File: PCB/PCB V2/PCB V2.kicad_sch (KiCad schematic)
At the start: 57 parts, among them J1 Screw_Terminal_01x03, J2 Screw_Terminal_01x03, J3 USB_B, J4 Conn_01x02_Pin, K1 Relay_SPDT, K2 Relay_SPDT, Q1 S8050, Q2 S8050, Q3 S8050, SW1 On/Off, SW2 SW_Push, SW3 SW_Push, U1 LM317_TO-220, U2 LM317_TO-220

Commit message: Cambiado el footprint del capacitor
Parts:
- C1, C4: footprint Capacitor_THT:CP_Radial_D10.0mm_P3.50mm -> Capacitor_THT:CP_Radial_D6.3mm_P2.50mm
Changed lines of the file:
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@@
 			)
 		)
-		(property "Footprint" "Capacitor_THT:CP_Radial_D10.0mm_P3.50mm"
+		(property "Footprint" "Capacitor_THT:CP_Radial_D6.3mm_P2.50mm"
 			(at 227.0252 110.49 0)
 			(effects
@@
 			)
 		)
-		(property "Footprint" "Capacitor_THT:CP_Radial_D10.0mm_P3.50mm"
+		(property "Footprint" "Capacitor_THT:CP_Radial_D6.3mm_P2.50mm"
 			(at 224.4852 80.01 0)
 			(effects

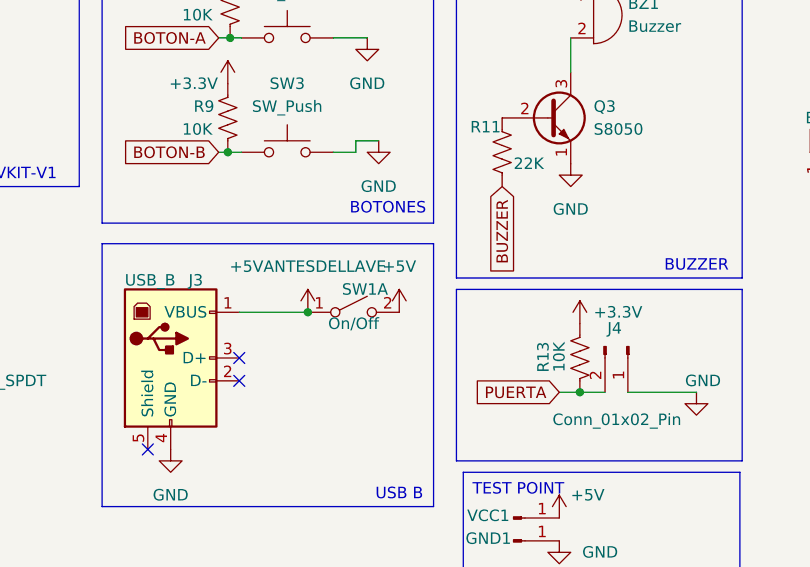
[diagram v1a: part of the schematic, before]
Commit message: .
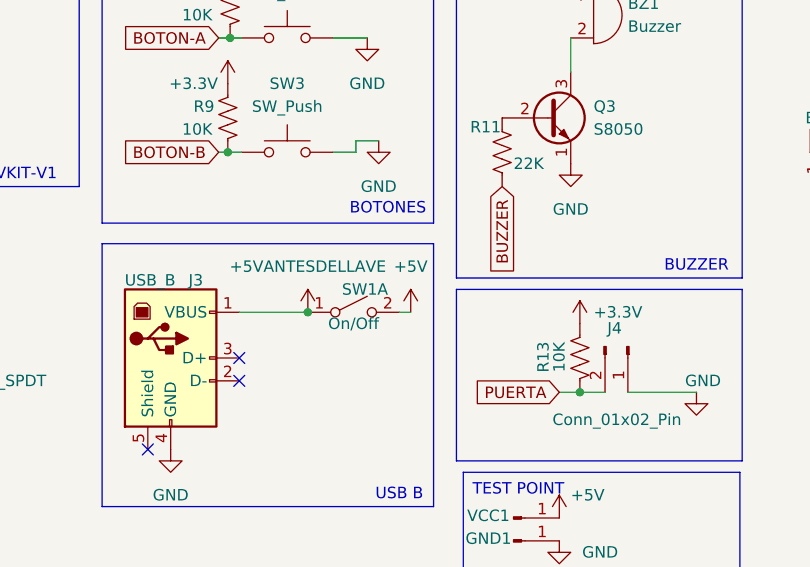
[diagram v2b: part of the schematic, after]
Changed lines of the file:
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@@
 	(wire
 		(pts
+			(xy 175.26 105.41) (xy 173.99 105.41)
+		)
+		(stroke
+			(width 0)
+			(type default)
+		)
+	)
+	(wire
+		(pts
 			(xy 256.54 95.25) (xy 247.65 95.25)
 		)
@@
 	(symbol
 		(lib_id "power:+5V")
-		(at 173.99 105.41 0)
+		(at 175.26 105.41 0)
 		(unit 1)
 		(exclude_from_sim no)
@@
 		(fields_autoplaced yes)
 		(property "Reference" "#PWR026"
-			(at 173.99 109.22 0)
+			(at 175.26 109.22 0)
 			(effects
 				(font
@@
 		)
 		(property "Value" "+5V"
-			(at 173.99 100.33 0)
+			(at 175.26 100.33 0)
 			(effects
 				(font
@@
 		)
 		(property "Footprint" ""
-			(at 173.99 105.41 0)
+			(at 175.26 105.41 0)
 			(effects
 				(font
@@
 		)
 		(property "Datasheet" ""
-			(at 173.99 105.41 0)
+			(at 175.26 105.41 0)
 			(effects
 				(font
@@
 		)
 		(property "Description" "Power symbol creates a global label with name \"+5V\""
-			(at 173.99 105.41 0)
+			(at 175.26 105.41 0)
 			(effects
 				(font

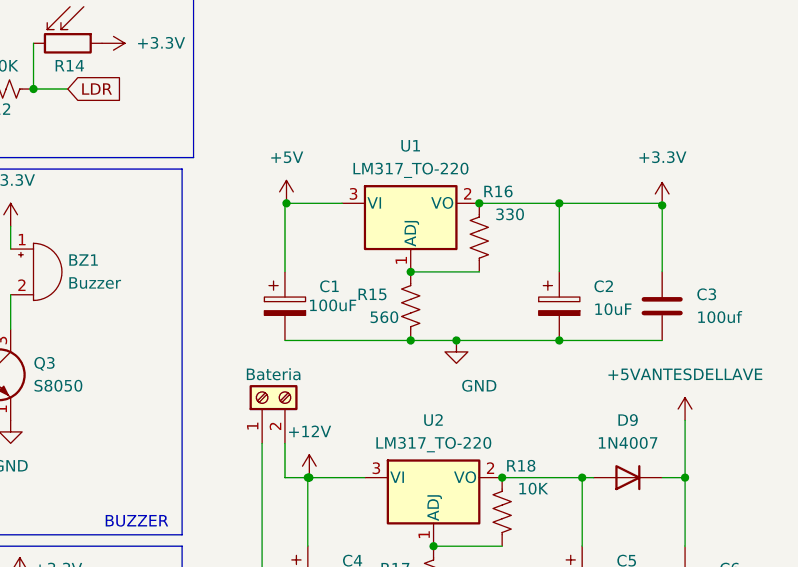
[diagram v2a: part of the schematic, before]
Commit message: .
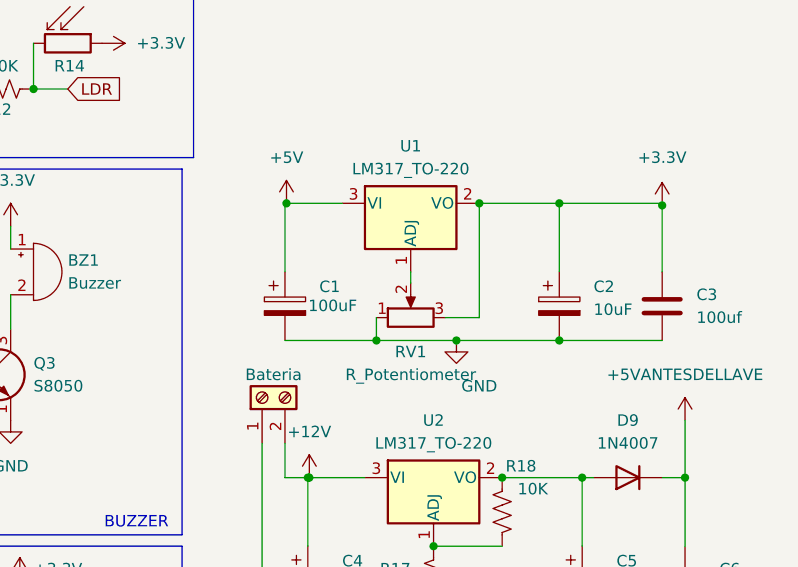
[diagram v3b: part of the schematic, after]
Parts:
- removed R15: 560, Resistor_THT:R_Axial_DIN0207_L6.3mm_D2.5mm_P10.16mm_Horizontal, symbol Device:R_US
- removed R16: 330, Resistor_THT:R_Axial_DIN0207_L6.3mm_D2.5mm_P10.16mm_Horizontal, symbol Device:R_US
- added RV1: R_Potentiometer, Potentiometer_THT:Potentiometer_Bourns_3386W_Horizontal, symbol Device:R_Potentiometer
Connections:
- net +3.3V: now also RV1.3
- net GND: now also RV1.1
- net at U1.1 (ADJ): now also RV1.2
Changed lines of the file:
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@@
 	)
 	(junction
+		(at 233.68 80.01)
+		(diameter 0)
+		(color 0 0 0 0)
+	)
+	(junction
 		(at 45.72 118.11)
 		(diameter 0)
@@
 	)
 	(junction
-		(at 245.11 64.77)
-		(diameter 0)
-		(color 0 0 0 0)
-	)
-	(junction
 		(at 97.79 119.38)
 		(diameter 0)
@@
 	)
 	(junction
-		(at 237.49 72.39)
-		(diameter 0)
-		(color 0 0 0 0)
-	)
-	(junction
 		(at 247.65 95.25)
 		(diameter 0)
@@
 	)
 	(junction
-		(at 237.49 80.01)
+		(at 245.11 64.77)
 		(diameter 0)
 		(color 0 0 0 0)
@@
 	(wire
 		(pts
+			(xy 233.68 80.01) (xy 242.57 80.01)
+		)
+		(stroke
+			(width 0)
+			(type default)
+		)
+	)
+	(wire
+		(pts
 			(xy 165.2503 28.535) (xy 157.6303 28.535)
 		)
@@
 	(wire
 		(pts
-			(xy 237.49 80.01) (xy 242.57 80.01)
+			(xy 223.52 80.01) (xy 233.68 80.01)
 		)
 		(stroke
@@
 	(wire
 		(pts
-			(xy 223.52 80.01) (xy 237.49 80.01)
-		)
-		(stroke
-			(width 0)
-			(type default)
-		)
-	)
-	(wire
-		(pts
 			(xy 166.5203 31.075) (xy 165.2503 31.075)
 		)
@@
 	(wire
 		(pts
-			(xy 237.49 72.39) (xy 245.11 72.39)
-		)
-		(stroke
-			(width 0)
-			(type default)
-		)
-	)
-	(wire
-		(pts
 			(xy 60.96 118.11) (xy 66.04 118.11)
 		)
@@
 	(wire
 		(pts
+			(xy 245.11 64.77) (xy 245.11 77.47)
+		)
+		(stroke
+			(width 0)
+			(type default)
+		)
+	)
+	(wire
+		(pts
+			(xy 237.49 73.66) (xy 237.49 72.39)
+		)
+		(stroke
+			(width 0)
+			(type default)
+		)
+	)
+	(wire
+		(pts
+			(xy 233.68 77.47) (xy 233.68 80.01)
+		)
+		(stroke
+			(width 0)
+			(type default)
+		)
+	)
+	(wire
+		(pts
+			(xy 241.3 77.47) (xy 245.11 77.47)
+		)
+		(stroke
+			(width 0)
+			(type default)
+		)
+	)
+	(wire
+		(pts
 			(xy 223.686 64.77) (xy 223.52 64.77)
 		)
@@
 	)
 	(symbol
-		(lib_id "Device:R_US")
-		(at 237.49 76.2 0)
-		(mirror y)
-		(unit 1)
-		(exclude_from_sim no)
-		(in_bom yes)
-		(on_board yes)
-		(dnp no)
-		(property "Reference" "R15"
-			(at 234.95 74.9299 0)
-			(effects
-				(font
-					(size 1.27 1.27)
-				)
-				(justify left)
-			)
-		)
-		(property "Value" "560"
-			(at 236.22 77.47 0)
-			(effects
-				(font
-					(size 1.27 1.27)
-				)
-				(justify left)
-			)
-		)
-		(property "Footprint" "Resistor_THT:R_Axial_DIN0207_L6.3mm_D2.5mm_P10.16mm_Horizontal"
-			(at 236.474 76.454 90)
-			(effects
-				(font
-					(size 1.27 1.27)
-				)
-				(hide yes)
-			)
-		)
-		(property "Datasheet" "~"
-			(at 237.49 76.2 0)
-			(effects
-				(font
-					(size 1.27 1.27)
-				)
-				(hide yes)
-			)
-		)
-		(property "Description" "Resistor, US symbol"
-			(at 237.49 76.2 0)
-			(effects
-				(font
-					(size 1.27 1.27)
-				)
-				(hide yes)
-			)
-		)
-		(pin "2"
-		)
-		(pin "1"
-		)
-		(instances
-			(project "PCB V2"
-				(path "/9d3c0d60-bbc5-4e33-843b-0a3b234644e7"
-					(reference "R15")
-					(unit 1)
-				)
-			)
-		)
-	)
-	(symbol
 		(lib_id "power:GND")
 		(at 207.01 114.3 0)
@@
 	)
 	(symbol
-		(lib_id "Device:LED")
-		(at 88.9 107.95 90)
+		(lib_id "Device:R_Potentiometer")
+		(at 237.49 77.47 90)
 		(unit 1)
 		(exclude_from_sim no)
@@
 		(on_board yes)
 		(dnp no)
-		(property "Reference" "D7"
-			(at 83.82 108.2675 90)
+		(fields_autoplaced yes)
+		(property "Reference" "RV1"
+			(at 237.49 81.28 90)
 			(effects
 				(font
 					(size 1.27 1.27)
 				)
-				(justify right)
 			)
 		)
-		(property "Value" "LED"
-			(at 83.82 110.8075 90)
+		(property "Value" "R_Potentiometer"
+			(at 237.49 83.82 90)
 			(effects
 				(font
 					(size 1.27 1.27)
 				)
-				(justify right)
 			)
 		)
-		(property "Footprint" "LED_THT:LED_D5.0mm_Clear"
-			(at 88.9 107.95 0)
+		(property "Footprint" "Potentiometer_THT:Potentiometer_Bourns_3386W_Horizontal"
+			(at 237.49 77.47 0)
 			(effects
 				(font
@@
 		)
 		(property "Datasheet" "~"
-			(at 88.9 107.95 0)
+			(at 237.49 77.47 0)
 			(effects
 				(font
@@
 			)
 		)
-		(property "Description" "Light emitting diode"
-			(at 88.9 107.95 0)
+		(property "Description" "Potentiometer"
+			(at 237.49 77.47 0)
 			(effects
 				(font
@@
 			)
 		)
+		(pin "1"
+		)
 		(pin "2"
 		)
-		(pin "1"
+		(pin "3"
 		)
 		(instances
 			(project "PCB V2"
 				(path "/9d3c0d60-bbc5-4e33-843b-0a3b234644e7"
-					(reference "D7")
+					(reference "RV1")
 					(unit 1)
 				)
@@
 	)
 	(symbol
-		(lib_id "power:+5V")
-		(at 175.26 105.41 0)
+		(lib_id "Device:LED")
+		(at 88.9 107.95 90)
 		(unit 1)
 		(exclude_from_sim no)
@@
 		(on_board yes)
 		(dnp no)
-		(fields_autoplaced yes)
-		(property "Reference" "#PWR026"
-			(at 175.26 109.22 0)
+		(property "Reference" "D7"
+			(at 83.82 108.2675 90)
 			(effects
 				(font
 					(size 1.27 1.27)
 				)
-				(hide yes)
+				(justify right)
 			)
 		)
-		(property "Value" "+5V"
-			(at 175.26 100.33 0)
+		(property "Value" "LED"
+			(at 83.82 110.8075 90)
 			(effects
 				(font
 					(size 1.27 1.27)
 				)
+				(justify right)
 			)
 		)
-		(property "Footprint" ""
-			(at 175.26 105.41 0)
+		(property "Footprint" "LED_THT:LED_D5.0mm_Clear"
+			(at 88.9 107.95 0)
 			(effects
 				(font
@@
 			)
 		)
-		(property "Datasheet" ""
-			(at 175.26 105.41 0)
+		(property "Datasheet" "~"
+			(at 88.9 107.95 0)
 			(effects
 				(font
@@
 			)
 		)
-		(property "Description" "Power symbol creates a global label with name \"+5V\""
-			(at 175.26 105.41 0)
+		(property "Description" "Light emitting diode"
+			(at 88.9 107.95 0)
 			(effects
 				(font
@@
 			)
 		)
+		(pin "2"
+		)
 		(pin "1"
 		)
@@
 			(project "PCB V2"
 				(path "/9d3c0d60-bbc5-4e33-843b-0a3b234644e7"
-					(reference "#PWR026")
+					(reference "D7")
 					(unit 1)
 				)
@@
 	)
 	(symbol
-		(lib_id "Device:R_US")
-		(at 245.11 68.58 0)
-		(mirror x)
+		(lib_id "power:+5V")
+		(at 175.26 105.41 0)
 		(unit 1)
 		(exclude_from_sim no)
@@
 		(on_board yes)
 		(dnp no)
-		(property "Reference" "R16"
-			(at 248.92 63.5 0)
+		(fields_autoplaced yes)
+		(property "Reference" "#PWR026"
+			(at 175.26 109.22 0)
 			(effects
 				(font
 					(size 1.27 1.27)
 				)
-				(justify right)
+				(hide yes)
 			)
 		)
-		(property "Value" "330"
-			(at 250.19 66.04 0)
+		(property "Value" "+5V"
+			(at 175.26 100.33 0)
 			(effects
 				(font
 					(size 1.27 1.27)
 				)
-				(justify right)
 			)
 		)
-		(property "Footprint" "Resistor_THT:R_Axial_DIN0207_L6.3mm_D2.5mm_P10.16mm_Horizontal"
-			(at 246.126 68.326 90)
+		(property "Footprint" ""
+			(at 175.26 105.41 0)
 			(effects
 				(font
@@
 			)
 		)
-		(property "Datasheet" "~"
-			(at 245.11 68.58 0)
+		(property "Datasheet" ""
+			(at 175.26 105.41 0)
 			(effects
 				(font
@@
 			)
 		)
-		(property "Description" "Resistor, US symbol"
-			(at 245.11 68.58 0)
+		(property "Description" "Power symbol creates a global label with name \"+5V\""
+			(at 175.26 105.41 0)
 			(effects
 				(font
@@
 			)
 		)
-		(pin "2"
-		)
 		(pin "1"
 		)
@@
 			(project "PCB V2"
 				(path "/9d3c0d60-bbc5-4e33-843b-0a3b234644e7"
-					(reference "R16")
+					(reference "#PWR026")
 					(unit 1)
 				)
